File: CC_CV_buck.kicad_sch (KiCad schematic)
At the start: 29 parts, among them Q1 TIP42C, Q2 AO3400A, Q3 MMBT3906, U1 OPA2197xD, U2 INA194, U3 AOZ6605PI-1

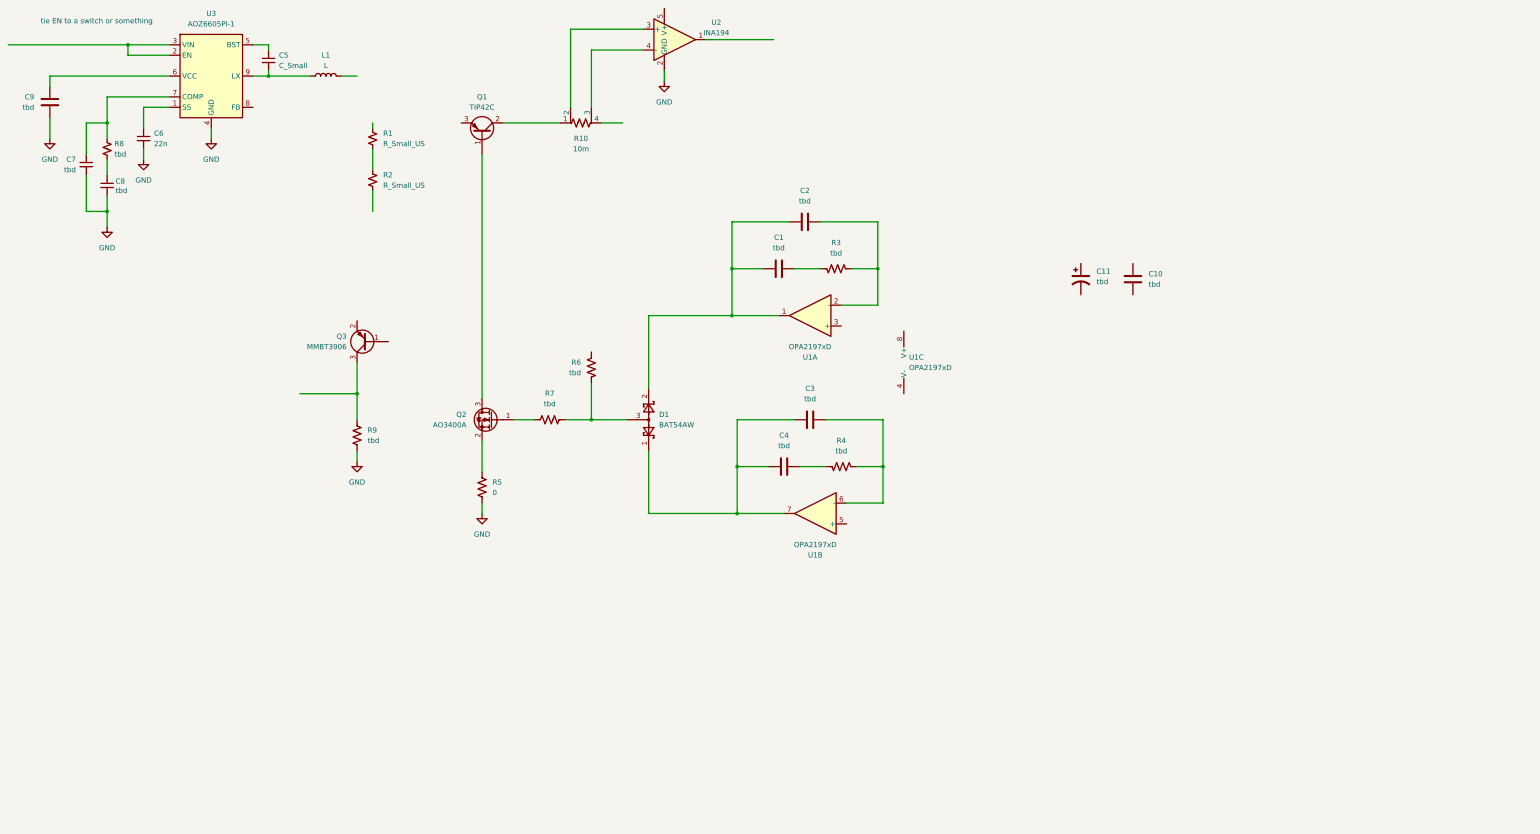
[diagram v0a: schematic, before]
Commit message: did a bunch of stuff
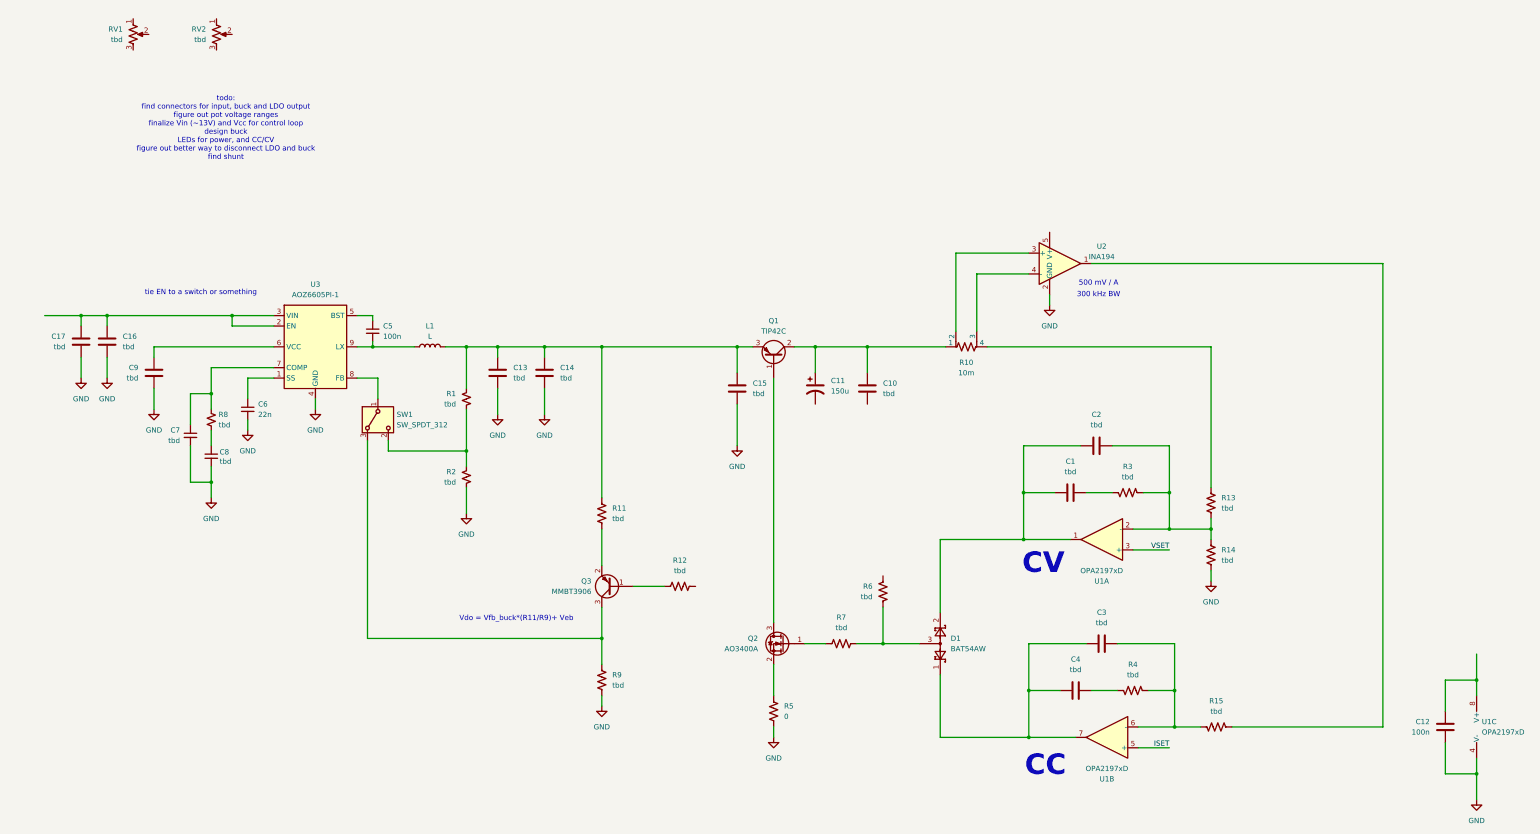
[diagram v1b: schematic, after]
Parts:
- added C12: 100n, symbol Device:C
- added C13, C14, C15, C16, C17: tbd, symbol Device:C
- added R11, R12, R13, R14, R15: tbd, symbol Device:R_US
- added RV1, RV2: tbd, symbol Device:R_Potentiometer_US
- added SW1: SW_SPDT_312, symbol Switch:SW_SPDT_312
- C11: value tbd -> 150u
- C5: value C_Small -> 100n
- R1, R2: value R_Small_US -> tbd
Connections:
- net GND: now also R2.2, U1.4 (V-), C12.2, C13.2, C14.2, C15.2, C16.2, C17.2, R14.1
- net at C2.1, R3.1, U1.2 (-): now also R13.1, R14.2
- net at Q1.2 (C), R10.1: now also C10.1, C11.1
- net at Q1.3 (E): now also L1.2, R1.1, C13.1, C14.1, C15.1, R11.1
- net VSET: now reaches U1.3 (+)
- net at R1.2, R2.1: now also SW1.2 (C)
- net at U3.2 (EN), U3.3 (VIN): now also C16.1, C17.1
- net at U3.8 (FB): now also SW1.1 (B)
- net ISET: now reaches U1.5 (+)
- net at C3.1, R4.1, U1.6 (-): now also R15.2
- net at Q3.1 (B): now also R12.1
- net at Q3.2 (E): now also R11.2
- net at Q3.3 (C), R9.1: now also SW1.3 (A)
- net at U2.1: now also R15.1
- net at R10.4: now also R13.2
- net at U1.8 (V+): now also C12.1
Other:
- note added: "300 kHz BW"
- note added: "500 mV / A"
- note added: "CC"
- note added: "CV"
- note added: "Vdo = Vfb_buck*(R11/R9)+ Veb"
- note added: "todo: find connectors for input, buck and LDO output figure out pot voltage ranges finalize Vin (~13V) and Vcc for control loop design buck LEDs for power, and CC/CV figure out better way to disconnect LDO and buck find shunt"
- moved on the sheet: C1, C10, C11, C2, C3, C4, C5, C6, C7, C8, C9, D1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
